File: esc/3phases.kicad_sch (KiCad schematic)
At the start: 44 parts, among them U2 GS8051, U3 GS8051

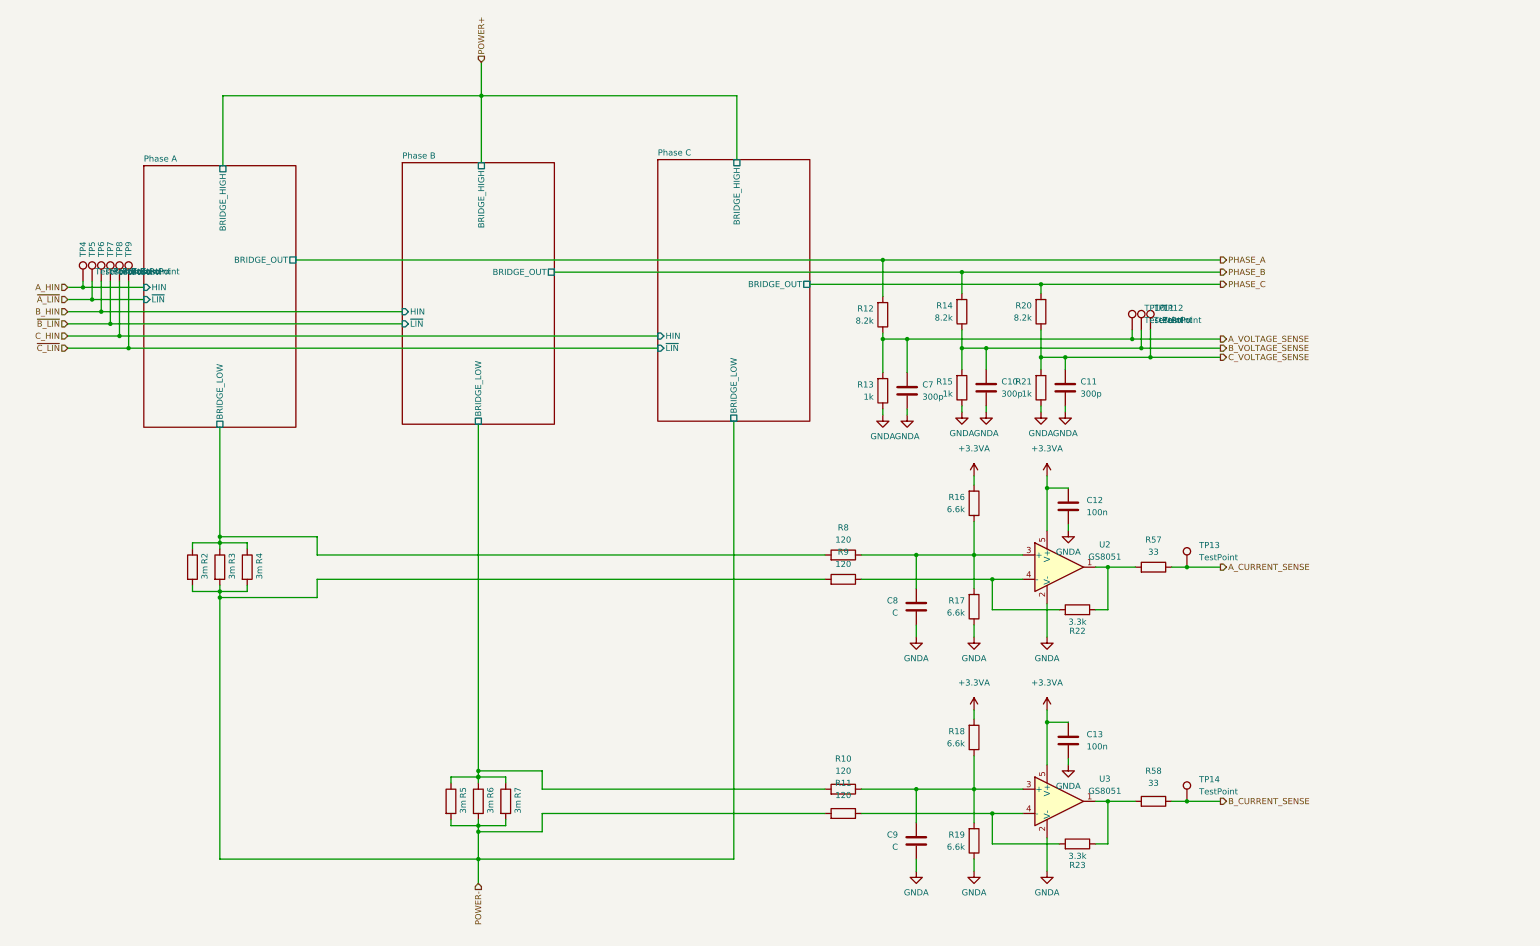
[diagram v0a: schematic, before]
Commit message: Some stuff
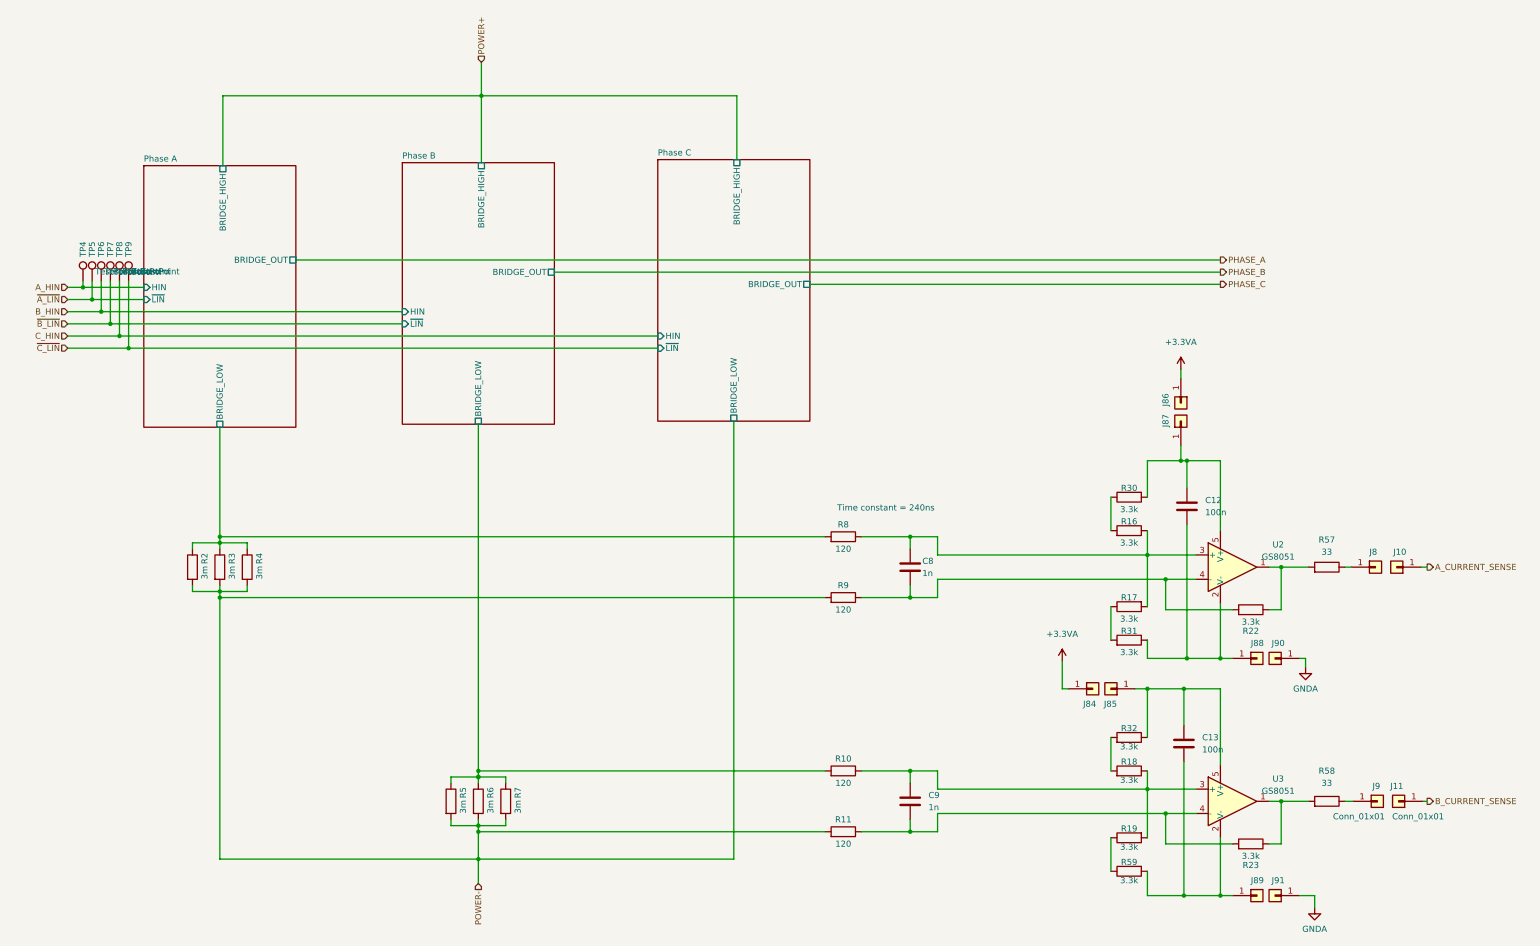
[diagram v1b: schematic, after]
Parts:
- removed C10, C11, C7: 300p, Capacitor_SMD:C_0603_1608Metric, symbol Device:C
- removed R12, R14, R20: 8.2k, Resistor_SMD:R_0603_1608Metric, symbol Device:R
- removed R13, R15, R21: 1k, Resistor_SMD:R_0603_1608Metric, symbol Device:R
- removed TP10, TP11, TP12, TP13, TP14: TestPoint, TestPoint:TestPoint_Pad_1.0x1.0mm, symbol Connector:TestPoint
- added J10, J11, J84, J86, J90, J91: Conn_01x01, Library:SmallPin, symbol Connector_Generic:Conn_01x01
- added J8, J85, J87, J88, J89, J9: Conn_01x01, Library:SmallPad, symbol Connector_Generic:Conn_01x01
- added R30, R31, R32, R59: 3.3k, Resistor_SMD:R_0603_1608Metric, symbol Device:R
- C8, C9: value C -> 1n
- R16, R17, R18, R19: value 6.6k -> 3.3k
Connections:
- net +3.3VA: now also J84.1 (Pin_1), J86.1 (Pin_1); no longer C12.1, C13.1, R16.2, R18.2, U2.5 (V+), U3.5 (V+)
- net A_CURRENT_SENSE: now also J10.1 (Pin_1); no longer R57.1
- net B_CURRENT_SENSE: now also J11.1 (Pin_1); no longer R58.1
- net GNDA: now also J90.1 (Pin_1), J91.1 (Pin_1); no longer C12.2, C13.2, C8.2, C9.2, R17.1, R19.1, U2.2 (V-), U3.2 (V-)
- net at R11.1, R23.2, U3.4 (-): now also C9.2
- net at R22.2, R9.1, U2.4 (-): now also C8.2
- new net: C12.2, J88.1 (Pin_1), R31.1, U2.2 (V-)
- new net: R17.1, R31.2
- new net: C13.1, J85.1 (Pin_1), R32.1, U3.5 (V+)
- new net: R16.2, R30.1
- new net: C12.1, J87.1 (Pin_1), R30.2, U2.5 (V+)
- new net: C13.2, J89.1 (Pin_1), R59.2, U3.2 (V-)
- new net: R19.1, R59.1
- new net: J8.1 (Pin_1), R57.1
- new net: J9.1 (Pin_1), R58.1
- new net: R18.2, R32.2
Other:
- note added: "Time constant = 240ns"
- moved on the sheet: C12, C13, C8, C9, R10, R11, R16, R17, R18, R19, R22, R23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

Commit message: Pretty much finished new design
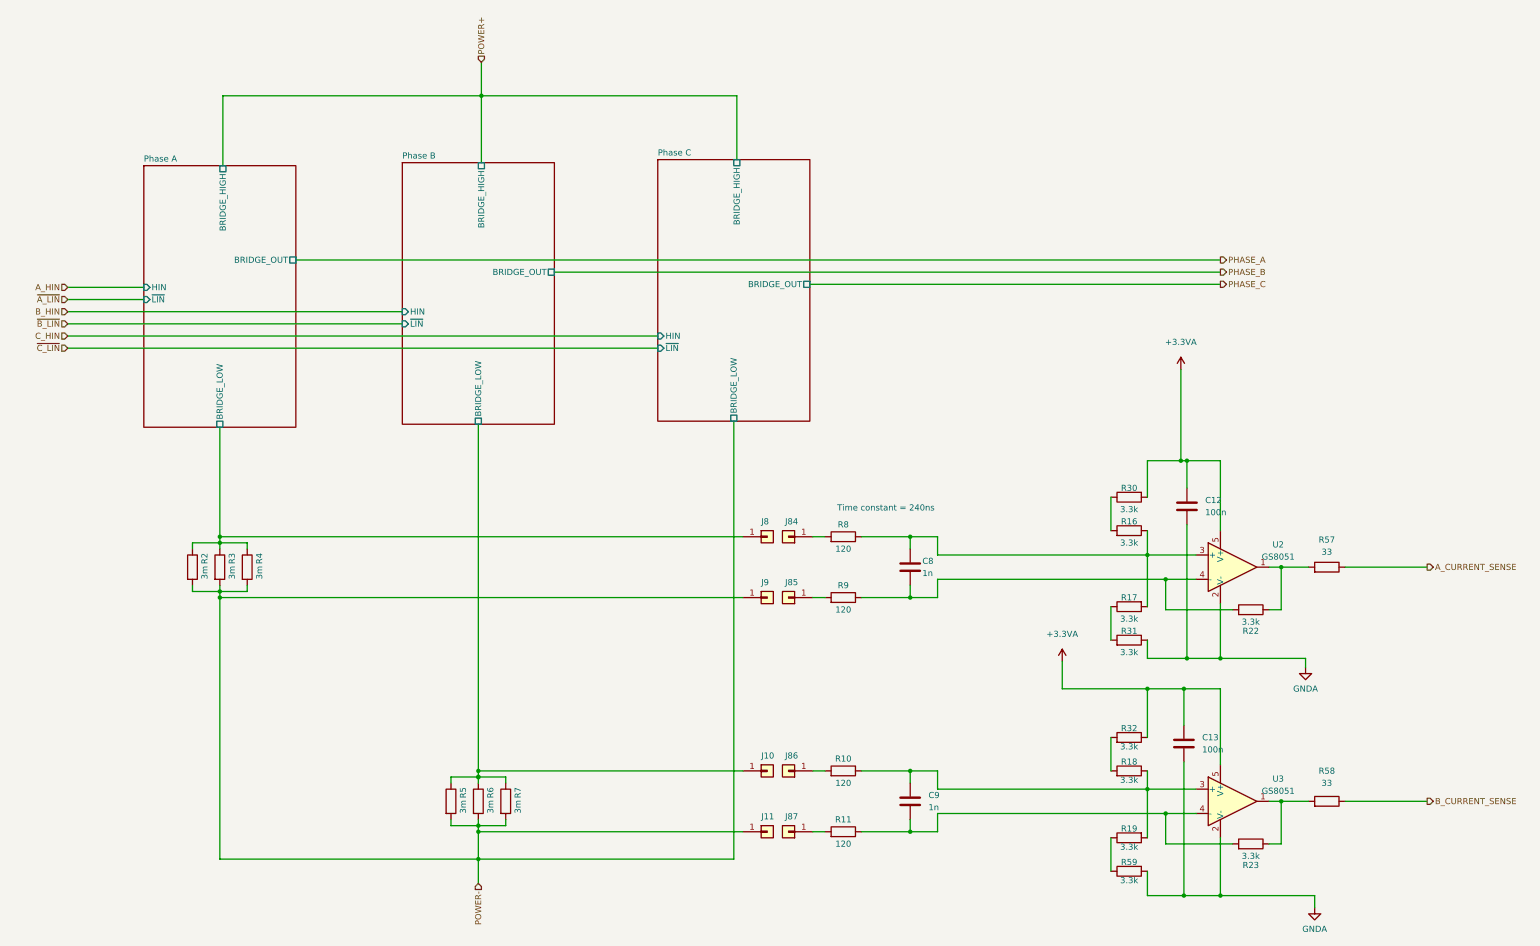
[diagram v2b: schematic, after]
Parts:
- removed J88, J89: Conn_01x01, Library:SmallPad, symbol Connector_Generic:Conn_01x01
- removed J90, J91: Conn_01x01, Library:SmallPin, symbol Connector_Generic:Conn_01x01
- removed TP4, TP5, TP6, TP7, TP8, TP9: TestPoint, TestPoint:TestPoint_Pad_1.0x1.0mm, symbol Connector:TestPoint
- J10, J11: footprint Library:SmallPin -> Library:SmallPad
- J85, J87: footprint Library:SmallPad -> Library:SmallPin
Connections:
- net +3.3VA: now also C12.1, C13.1, R30.2, R32.1, U2.5 (V+), U3.5 (V+); no longer J84.1 (Pin_1), J86.1 (Pin_1)
- net A_CURRENT_SENSE: now also R57.1; no longer J10.1 (Pin_1)
- net B_CURRENT_SENSE: now also R58.1; no longer J11.1 (Pin_1)
- net GNDA: now also C12.2, C13.2, R31.1, R59.2, U2.2 (V-), U3.2 (V-)
- net POWER-: now also J11.1 (Pin_1), J9.1 (Pin_1); no longer R11.2, R9.2
- net Phase A/BRIDGE_LOW: now also J8.1 (Pin_1); no longer R8.2
- net Phase B/BRIDGE_LOW: now also J10.1 (Pin_1); no longer R10.2
- new net: J84.1 (Pin_1), R8.2
- new net: J85.1 (Pin_1), R9.2
- new net: J86.1 (Pin_1), R10.2
- new net: J87.1 (Pin_1), R11.2
